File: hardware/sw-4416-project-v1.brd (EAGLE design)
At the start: 94 x 52.1 mm, 56 parts, among them IC1 MCP73831, U1 ADP3338, X1 USB-MICROB, Y1 16M

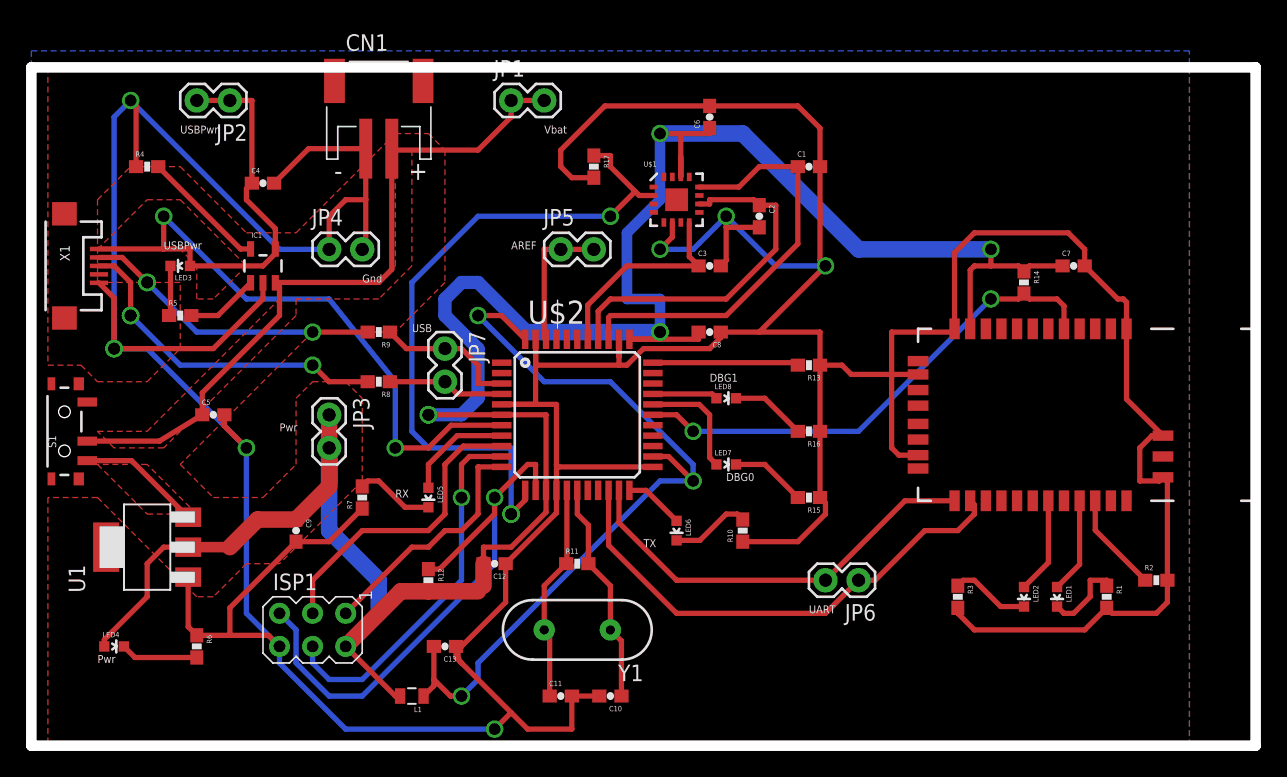
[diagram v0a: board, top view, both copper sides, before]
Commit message: working on embedded side code
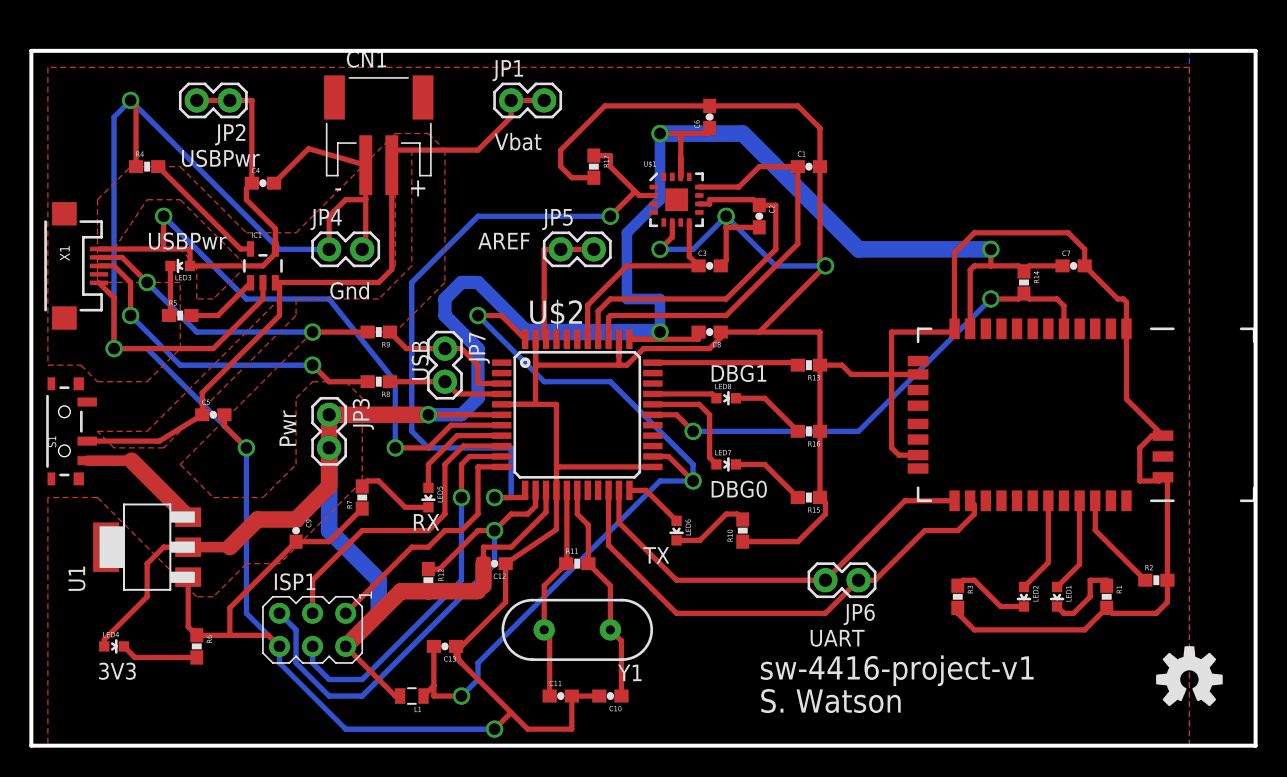
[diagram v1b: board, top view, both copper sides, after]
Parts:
- added U$4: (no value), SparkFun:OSHW-LOGO-M
- moved CN1 1.27 mm to (26.7, 74.9)
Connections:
- net N$11 renamed VIN
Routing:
- net MCU_RST: track 44.2 -> 38.8 mm
- net 3.3V: track 201.9 -> 200.3 mm
- net ST: track 53.3 -> 54.0 mm
- net GND: track 437.8 -> 437.2 mm
- added copper zone on layer 1, net GND
- removed copper zone on layer 1, net N$29
- removed copper zone on layer 1, net VIN
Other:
- board size 94 x 52.1 mm -> 94 x 53.3 mm
- board text added: "3V3"
- board text added: "S. Watson"
- board text added: "sw-4416-project-v1"
